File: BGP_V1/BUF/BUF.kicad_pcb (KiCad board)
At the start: 2 copper layers, 30 x 30 mm, 23 parts, among them P1 CONN_01X05, P2 CONN_01X02, P3 CONN_01X12, U1 MC33178, U2 TLV170

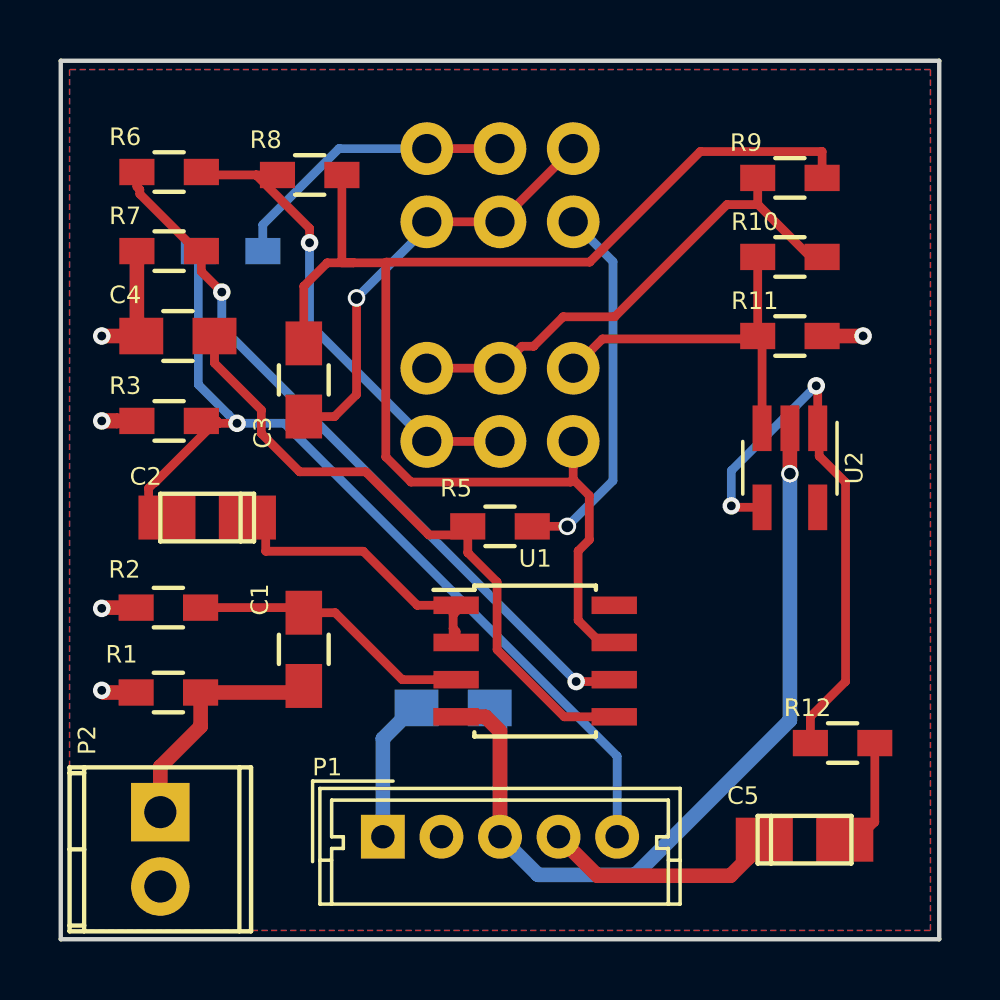
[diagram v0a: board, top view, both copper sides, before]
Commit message: some cleanup
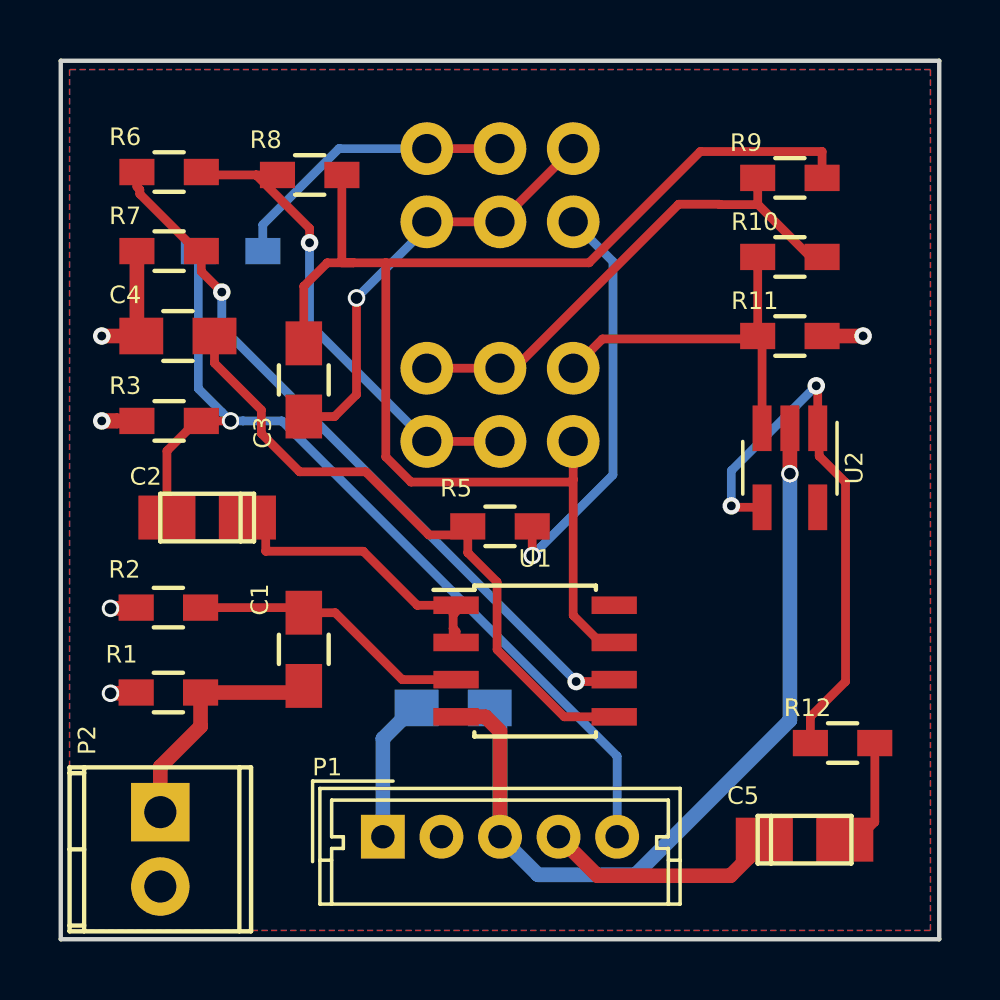
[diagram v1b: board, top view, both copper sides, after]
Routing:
- net /VF2_2: track 12.8 -> 14.1 mm
- net Earth: track 10.1 -> 9.51 mm
